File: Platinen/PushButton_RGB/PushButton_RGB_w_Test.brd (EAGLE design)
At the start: 100 x 80 mm, 149 parts, among them IC1 4017D, IC2 4011D, IC3 4017D

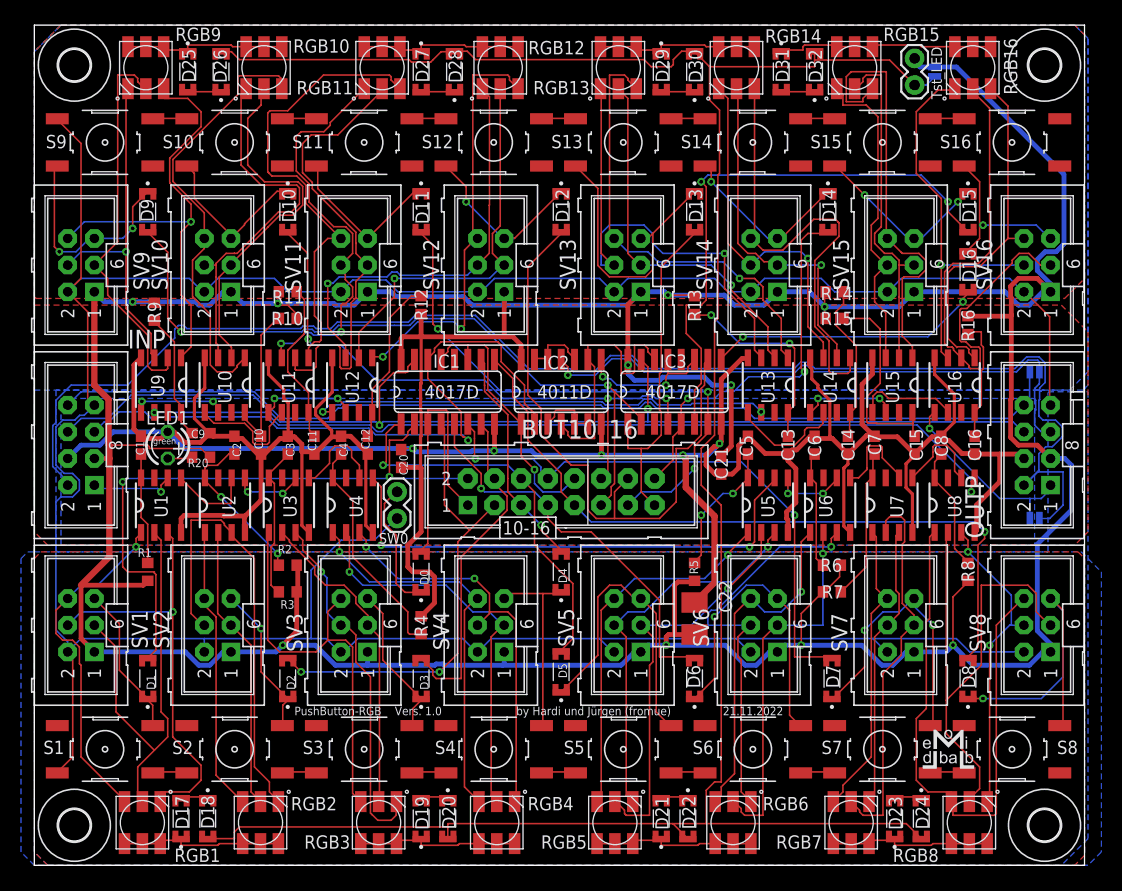
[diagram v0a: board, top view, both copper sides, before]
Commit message: First Version Push Button 16x RGB
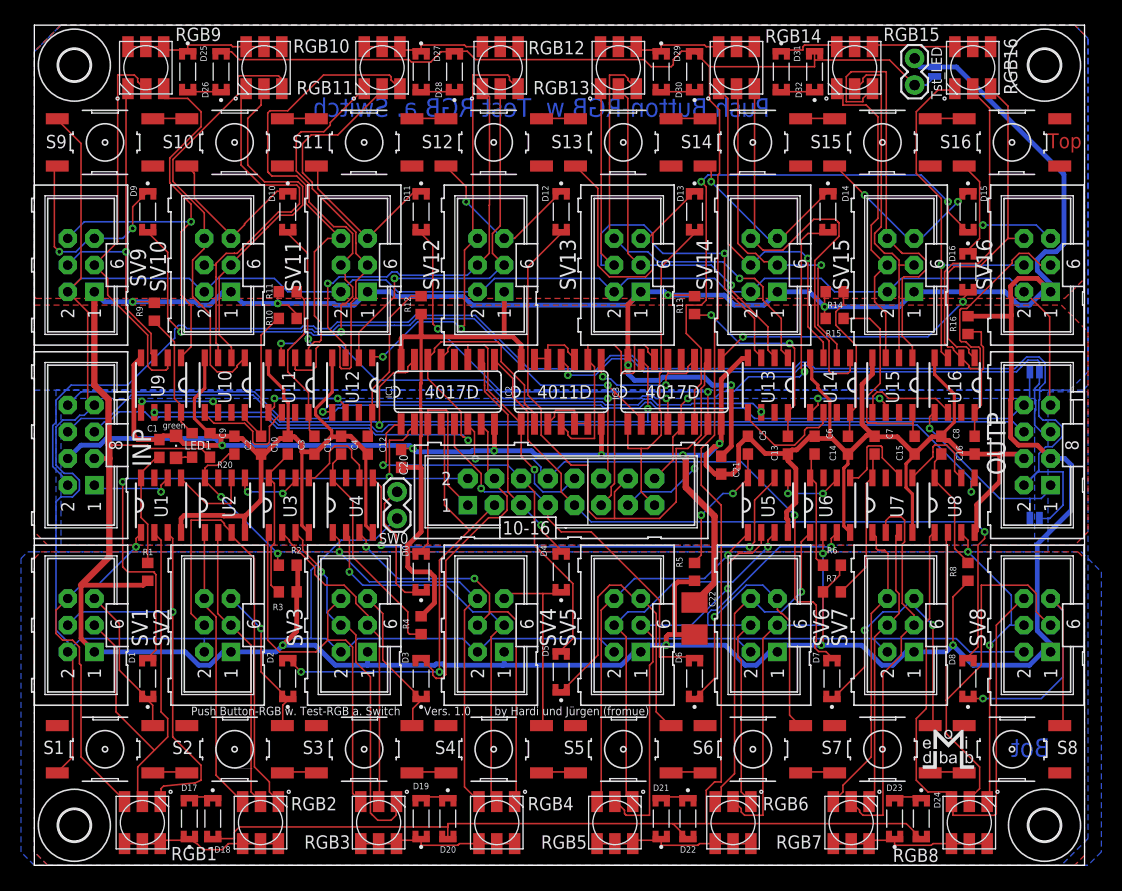
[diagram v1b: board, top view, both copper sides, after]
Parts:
- LED1: device led:LED3MM -> led:CHIPLED_0805
- moved C1 1.77 mm to (11.9, 39.7)
- moved LED1 0.81 mm to (13.5, 39.8), turned to 0 degrees
- moved D17 0.79 mm to (14.8, 4.45)
- moved D18 0.48 mm to (17.0, 4.45)
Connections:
- net GND: now also LED1.C; no longer LED1.K
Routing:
- net GND: track 288.4 -> 290.0 mm, vias 5 -> 6
- net N$21: track 2.39 -> 1.53 mm
- net N$71: track 39.1 -> 39.9 mm
- net +5V: track 462.1 -> 461.3 mm
- net N$17: track 54.9 -> 54.2 mm
- net N$76: track 10.6 -> 11.2 mm
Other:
- board text added: ">RELEASE_DATE"
- board text added: "Bot"
- board text added: "INPUT"
- board text added: "OUTPUT"
- board text added: "Push Button-RGB w. Test RGB a. Switch"
- board text added: "Push Button-RGB w. Test-RGB a. Switch"
- board text added: "Push Button-RGB w. Test-RGB a. Switch Vers. 1.0 by Hardi und Jürgen (fromue)"
- board text added: "Top"
- board text added: "green"
- board text removed: "+"
- board text removed: "21.11.2022"
- board text removed: "Push Button-RGB w. Test-RGB"
- board text removed: "PushButton-RGB Vers. 1.0"
